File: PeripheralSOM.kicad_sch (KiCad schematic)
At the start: 6 parts, among them J4 52465-2470

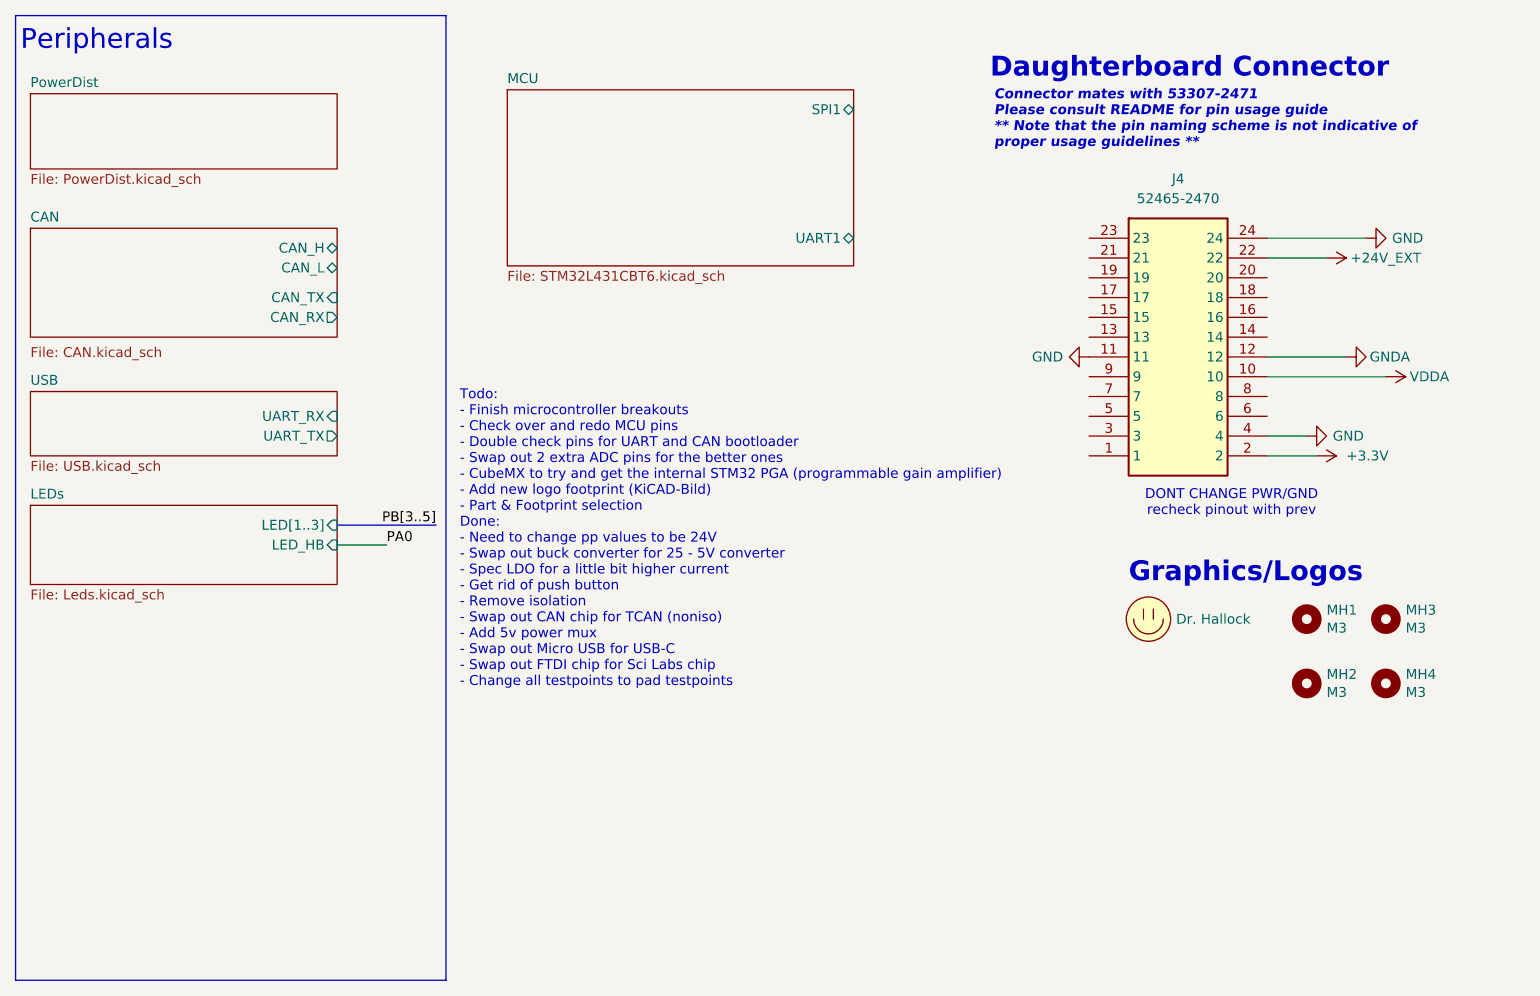
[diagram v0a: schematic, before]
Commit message: control but micro
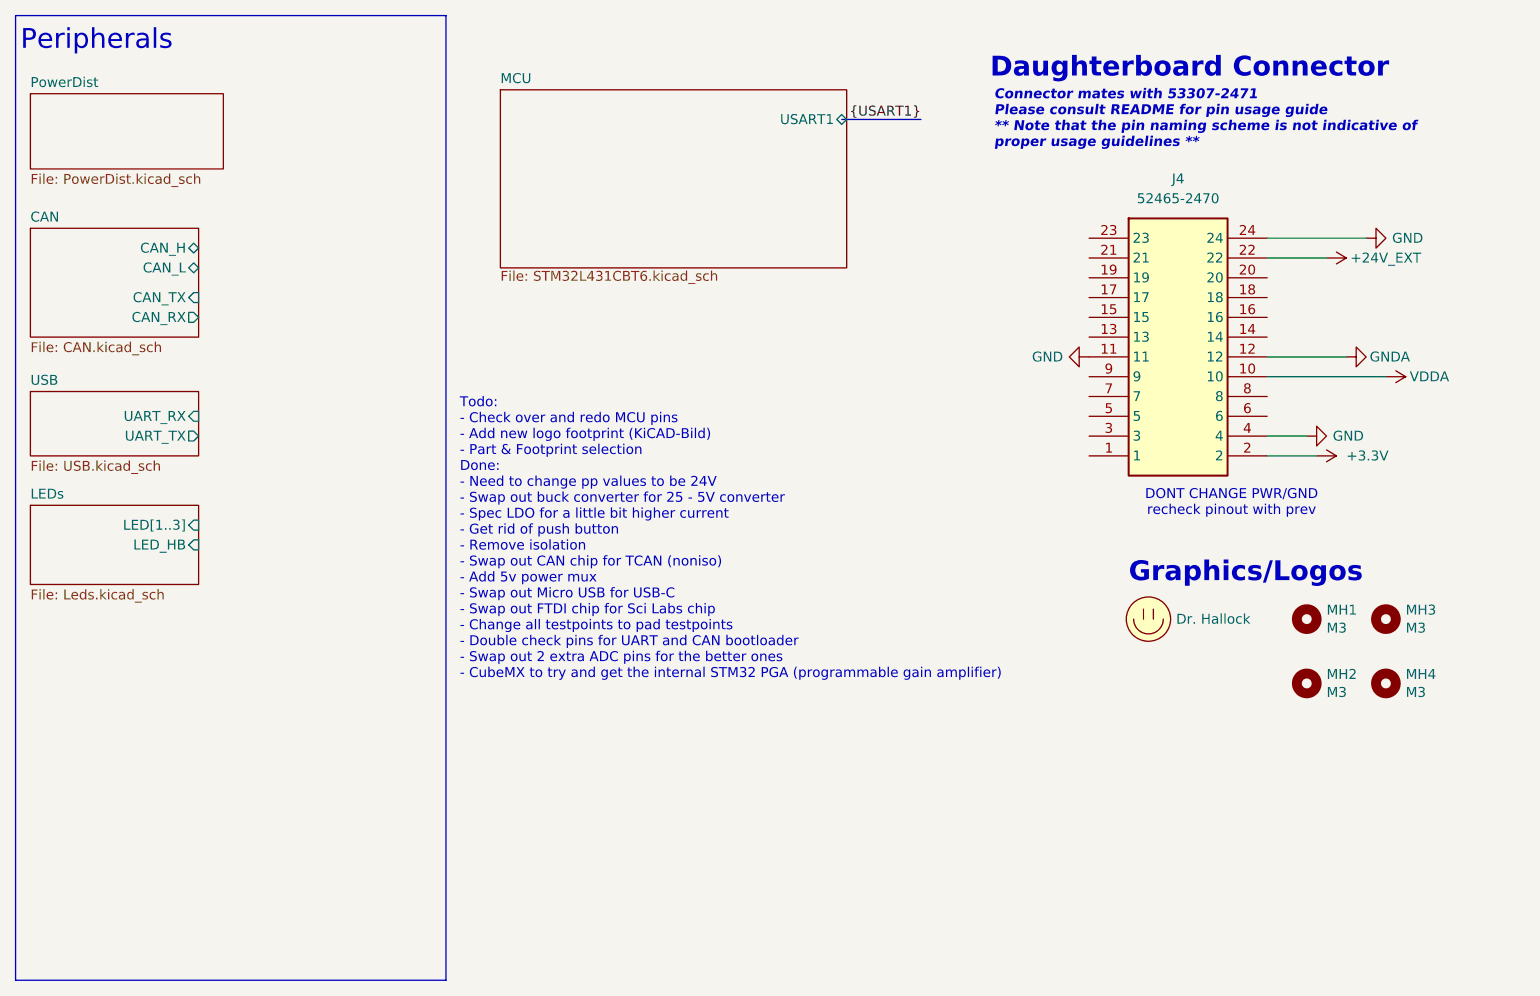
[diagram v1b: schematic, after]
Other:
- sheet MCU ports: added USART1; removed SPI1, UART1
- note added: "Todo: - Check over and redo MCU pins - Add new logo footprint (KiCAD-Bild) - Part & Footprint selection Done: - Need to change pp values to be 24V - Swap out buck converter for 25 - 5V converter - Spec LDO for a little bit higher current - Get rid of push button - Remove isolation - Swap out CAN chip for TCAN (noniso) - Add 5v power mux - Swap out Micro USB for USB-C - Swap out FTDI chip for Sci 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"
- note removed: "Todo: - Finish microcontroller breakouts - Check over and redo MCU pins - Double check pins for UART and CAN bootloader - Swap out 2 extra ADC pins for the better ones - CubeMX to try and get the internal STM32 PGA (programmable gain amplifier) - Add new logo footprint (KiCAD-Bild) - Part & Footprint selection Done: - Need to change pp values to be 24V - Swap out buck converter for 25 - 5V conver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"
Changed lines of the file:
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@@
 		)
 	)
-	(text "Todo:\n- Finish microcontroller breakouts\n- Check over and redo MCU pins\n- Double check pins for UART and CAN bootloader\n- Swap out 2 extra ADC pins for the better ones\n- CubeMX to try and get the internal STM32 PGA (programmable gain amplifier)\n- Add new logo footprint (KiCAD-Bild)\n- Part & Footprint selection\nDone:\n- Need to change pp values to be 24V\n- Swap out buck converter for 25 - 5V converter\n- Spec LDO for a little bit higher current\n- Get rid of push button\n- Remove isolation\n- Swap out CAN chip for TCAN (noniso)\n- Add 5v power mux\n- Swap out Micro USB for USB-C\n- Swap out FTDI chip for Sci Labs chip\n- Change all testpoints to pad testpoints\n"
+	(text "Todo:\n- Check over and redo MCU pins\n- Add new logo footprint (KiCAD-Bild)\n- Part & Footprint selection\nDone:\n- Need to change pp values to be 24V\n- Swap out buck converter for 25 - 5V converter\n- Spec LDO for a little bit higher current\n- Get rid of push button\n- Remove isolation\n- Swap out CAN chip for TCAN (noniso)\n- Add 5v power mux\n- Swap out Micro USB for USB-C\n- Swap out FTDI chip for Sci Labs chip\n- Change all testpoints to pad testpoints\n- Double check pins for UART and CAN bootloader\n- Swap out 2 extra ADC pins for the better ones\n- CubeMX to try and get the internal STM32 PGA (programmable gain amplifier)"
 		(exclude_from_sim no)
 		(at 69.088 79.248 0)
@@
 		)
 	)
-	(bus
+	(wire
 		(pts
-			(xy 53.34 77.47) (xy 66.04 77.47)
+			(xy 172.72 55.88) (xy 182.88 55.88)
 		)
 		(stroke
@@
 		)
 	)
-	(wire
+	(bus
 		(pts
-			(xy 172.72 55.88) (xy 182.88 55.88)
+			(xy 118.11 25.4) (xy 128.27 25.4)
 		)
 		(stroke
@@
 	(wire
 		(pts
-			(xy 59.69 80.01) (xy 53.34 80.01)
+			(xy 172.72 58.42) (xy 187.96 58.42)
 		)
 		(stroke
@@
 	(wire
 		(pts
-			(xy 172.72 58.42) (xy 187.96 58.42)
+			(xy 172.72 68.58) (xy 179.07 68.58)
 		)
 		(stroke
@@
 	(wire
 		(pts
-			(xy 172.72 68.58) (xy 179.07 68.58)
+			(xy 172.72 66.04) (xy 177.8 66.04)
 		)
 		(stroke
@@
 		)
 	)
-	(wire
-		(pts
-			(xy 172.72 66.04) (xy 177.8 66.04)
-		)
-		(stroke
-			(width 0)
-			(type default)
-		)
-	)
-	(label "PB[3..5]"
-		(at 66.04 77.47 180)
+	(label "{USART1}"
+		(at 128.27 25.4 180)
 		(effects
 			(font
@@
 			)
 			(justify right bottom)
-		)
-	)
-	(label "PA0"
-		(at 59.69 80.01 0)
-		(effects
-			(font
-				(size 1.27 1.27)
-			)
-			(justify left bottom)
 		)
 	)
@@
 	(sheet
 		(at 13.97 39.37)
-		(size 39.37 13.97)
+		(size 21.59 13.97)
 		(exclude_from_sim no)
 		(in_bom yes)
@@
 		)
 		(property "Sheetfile" "CAN.kicad_sch"
-			(at 13.97 54.5596 0)
+			(at 13.97 53.9246 0)
 			(effects
 				(font
@@
 		)
 		(pin "CAN_H" bidirectional
-			(at 53.34 41.91 0)
+			(at 35.56 41.91 0)
 			(effects
 				(font
@@
 		)
 		(pin "CAN_L" bidirectional
-			(at 53.34 44.45 0)
+			(at 35.56 44.45 0)
 			(effects
 				(font
@@
 		)
 		(pin "CAN_RX" output
-			(at 53.34 50.8 0)
+			(at 35.56 50.8 0)
 			(effects
 				(font
@@
 		)
 		(pin "CAN_TX" input
-			(at 53.34 48.26 0)
+			(at 35.56 48.26 0)
 			(effects
 				(font
@@
 	)
 	(sheet
-		(at 75.184 21.59)
-		(size 44.45 22.606)
+		(at 74.295 21.59)
+		(size 44.45 22.86)
 		(exclude_from_sim no)
 		(in_bom yes)
@@
 		)
 		(property "Sheetname" "MCU"
-			(at 75.184 20.8784 0)
+			(at 74.295 20.8784 0)
 			(effects
 				(font
@@
 		)
 		(property "Sheetfile" "STM32L431CBT6.kicad_sch"
-			(at 75.184 44.7806 0)
+			(at 74.295 44.7806 0)
 			(effects
 				(font
@@
 			)
 		)
-		(pin "UART1" bidirectional
-			(at 119.634 40.64 0)
-			(effects
-				(font
-					(size 1.27 1.27)
-				)
-				(justify right)
-			)
-		)
-		(pin "SPI1" bidirectional
-			(at 119.634 24.13 0)
+		(pin "USART1" bidirectional
+			(at 118.745 25.4 0)
 			(effects
 				(font
@@
 	(sheet
 		(at 13.97 74.93)
-		(size 39.37 10.16)
+		(size 21.59 10.16)
 		(exclude_from_sim no)
 		(in_bom yes)
@@
 		)
 		(pin "LED[1..3]" input
-			(at 53.34 77.47 0)
+			(at 35.56 77.47 0)
 			(effects
 				(font
@@
 		)
 		(pin "LED_HB" input
-			(at 53.34 80.01 0)
+			(at 35.56 80.01 0)
 			(effects
 				(font
@@
 	(sheet
 		(at 13.97 22.098)
-		(size 39.37 9.652)
+		(size 24.765 9.652)
 		(exclude_from_sim no)
 		(in_bom yes)
@@
 	(sheet
 		(at 13.97 60.325)
-		(size 39.37 8.255)
+		(size 21.59 8.255)
 		(exclude_from_sim no)
 		(in_bom yes)
@@
 		)
 		(pin "UART_RX" input
-			(at 53.34 63.5 0)
+			(at 35.56 63.5 0)
 			(effects
 				(font
@@
 		)
 		(pin "UART_TX" output
-			(at 53.34 66.04 0)
-			(effects
-				(font
+			(at 35.56 66.04 0)
+			(effects
+				(font
